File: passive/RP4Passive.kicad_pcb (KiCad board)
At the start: 2 copper layers, 30.4 x 59.4 mm, 8 parts, among them M1 Noctua

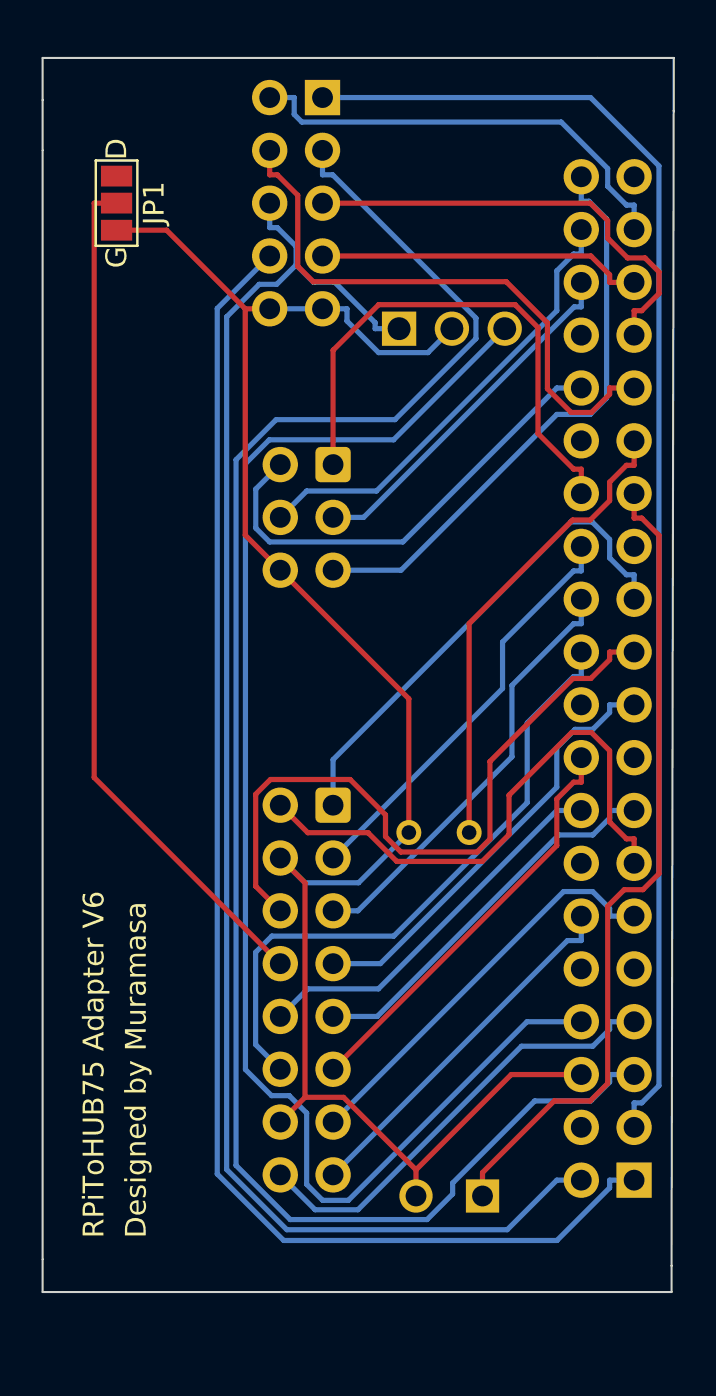
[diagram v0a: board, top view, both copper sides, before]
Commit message: version 7
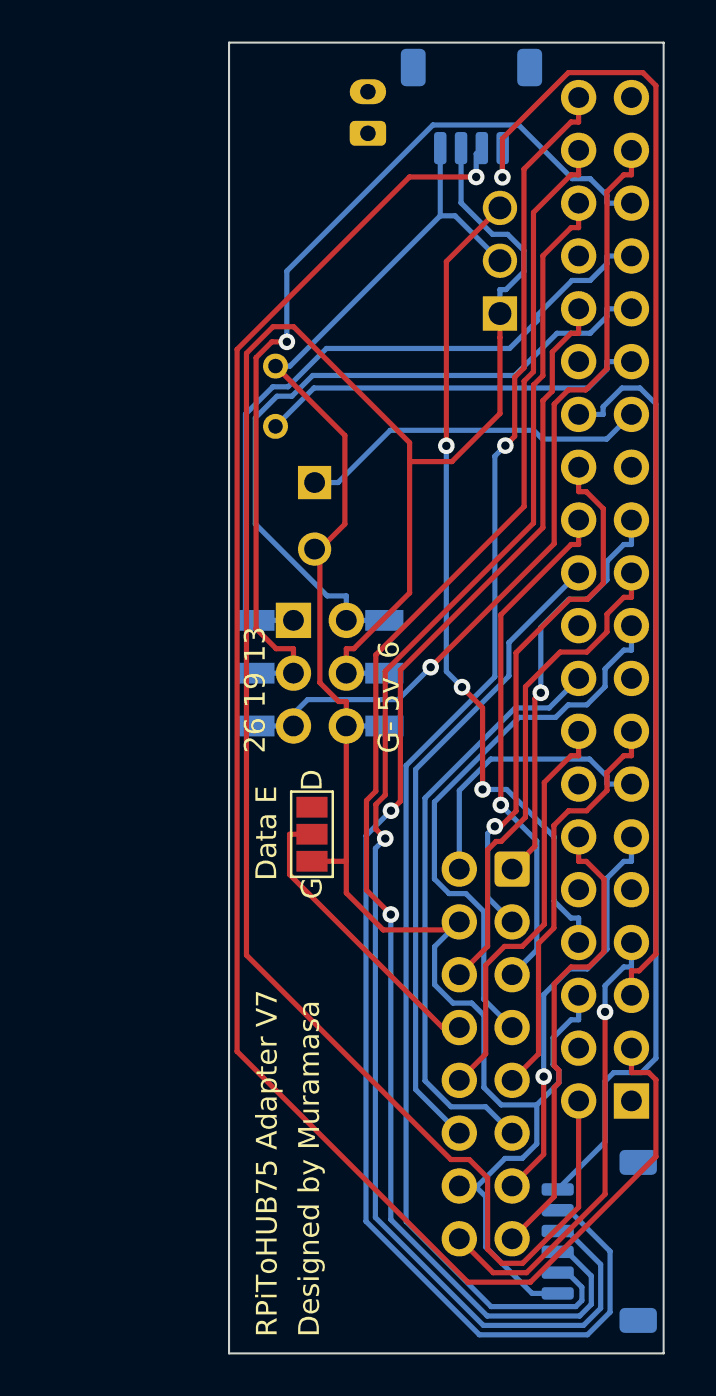
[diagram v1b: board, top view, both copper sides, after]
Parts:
- added J1: Conn_01x01, Custom:raspberrypi_2_3, B.Cu at (113.9, 81.5)
- added J2: Conn_01x02_Socket, Custom:JST_PH_S2B-PH-K_1x02_P2.00mm_Horizontal, B.Cu at (151.5, 59.1)
- added SCD30: Conn_01x04_Socket, Custom:STEMMA QT 1x04, B.Cu at (156.5, 57.8)
- GPIO1: value 02x05 -> 02x03; footprint Connector_PinHeader_2.54mm:PinHeader_2x05_P2.54mm_Horizontal -> Custom:GPIO Header
- HUB1: footprint Connector_IDC:IDC-Header_2x08_P2.54mm_Horizontal -> Custom:HUB75
- IO1: footprint Connector_IDC:IDC-Header_2x03_P2.54mm_Horizontal -> Custom:JST_SH_SM06B-SRSS-TB_1x06-1MP_P1.00mm_Horizontal
- RPiGPIO1: footprint Connector_PinSocket_2.54mm:PinSocket_2x20_P2.54mm_Vertical -> Custom:RPi GPIO
- moved IO1 39.5 mm to (162.7, 112.4), turned to -90 degrees
- moved BZ1 35.3 mm to (149.0, 75.9), turned to -90 degrees
- moved JP1 31.8 mm to (148.8, 92.8)
- moved GPIO1 27.7 mm to (149.2, 85.1)
- moved S1 21.6 mm to (147.1, 73.2), turned to 90 degrees
- moved HUB1 9.14 mm to (158.5, 94.5)
- moved M1 4.91 mm to (157.9, 67.8), turned to -90 degrees
- moved RPiGPIO1 3.81 mm to (164.2, 105.7)
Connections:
- GPIO1 pad 1: GPIO 2 -> GPIO 13
- GPIO1 pad 2: GPIO 26 -> GPIO 6
- GPIO1 pad 3: GPIO 3 -> GPIO 19
- GPIO1 pad 4: GPIO 6 -> 5v
- GPIO1 pad 5: GPIO 13 -> GPIO 26
- GPIO1 pad 6: 5v -> Net-(BZ1-+)
- RPiGPIO1 pad 1: 3.3v -> unconnected-(RPiGPIO1-Pin_1-Pad1)
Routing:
- net 3.3v: track 68.0 -> 0.00 mm
- net IO3: track 17.3 -> 71.6 mm, vias 0 -> 1
- net IO4: track 22.0 -> 71.6 mm, vias 0 -> 1
- net IO2: track 22.5 -> 69.1 mm, vias 0 -> 1
- net IO5: track 27.9 -> 70.1 mm, vias 0 -> 1
- net 5v: track 74.7 -> 105.6 mm
- net GPIO 19: track 15.7 -> 44.7 mm, vias 0 -> 1
- net FAN: track 68.6 -> 39.9 mm, vias 0 -> 3
- net GPIO 3: track 83.9 -> 56.7 mm, vias 0 -> 1
- net Net-(HUB1-Pin_8): track 41.4 -> 14.2 mm
- net BUZZ: track 39.6 -> 16.9 mm
- net IO1: track 25.8 -> 45.3 mm
- net GPIO 2: track 64.5 -> 83.6 mm, vias 0 -> 1
- net GPIO 26: track 21.8 -> 39.8 mm, vias 0 -> 1
- net G1: track 27.1 -> 13.4 mm
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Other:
- board size 30.4 x 59.4 mm -> 20.9 x 63 mm
- board text added: "26 19 13 G- 5v 6"
- board text added: "RPiToHUB75 Adapter V7"
- board text removed: "RPiToHUB75 Adapter V6"

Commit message: update image
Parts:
- J2: value Conn_01x02_Socket -> 1x02
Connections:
- J2 pad 1: unconnected-(J2-Pin_1-Pad1) -> 5v
- J2 pad 2: unconnected-(J2-Pin_2-Pad2) -> Net-(BZ1-+)
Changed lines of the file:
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@@
   (net 41 "5v")
   (net 42 "unconnected-(RPiGPIO1-Pin_1-Pad1)")
-  (net 43 "unconnected-(J2-Pin_1-Pad1)")
-  (net 44 "unconnected-(J2-Pin_2-Pad2)")
   (footprint "Jumper:SolderJumper-3_P1.3mm_Open_Pad1.0x1.5mm_NumberLabels" (layer "F.Cu")
     (at 148.844 92.837 -90)
@@
       (stroke (width 0.05) (type default)) (fill none) (layer "B.CrtYd"))
     (model "C:/Users/Admin/Downloads/RASPBERRY_PI_5.STEP/RASPBERRY_PI_5.STEP"
-      (offset (xyz 10 -24.5 12.5))
+      (opacity 0.0000)      (offset (xyz 10 -24.5 12.5))
       (scale (xyz 1 1 1))
       (rotate (xyz 90 0 0))
     )
     (model "C:/Users/Admin/Downloads/black-aluminum-heatsink-for-raspberry-pi-1.snapshot.3/Heat sink Al.step"
-      (offset (xyz 0.5 -19 7.5))
+      (opacity 0.0000)      (offset (xyz 0.5 -19 7.5))
       (scale (xyz 1 1 1))
       (rotate (xyz 90 0 0))
@@
         (effects (font (size 1 1) (thickness 0.15)) (justify mirror))
     )
-    (fp_text value "Conn_01x02_Socket" (at 1 -7.45 90) (layer "B.Fab") hide
+    (fp_text value "1x02" (at 1 -7.45 90) (layer "B.Fab") hide
         (effects (font (size 1 1) (thickness 0.15)) (justify mirror))
     )
@@
       (stroke (width 0.1) (type solid)) (layer "B.Fab"))
     (pad "1" thru_hole roundrect (at 0 0 90) (size 1.2 1.75) (drill 0.75) (layers "*.Cu" "*.Mask") (roundrect_rratio 0.208333)
-      (net 43 "unconnected-(J2-Pin_1-Pad1)") (pinfunction "Pin_1") (pintype "passive+no_connect"))
+      (net 41 "5v") (pinfunction "Pin_1") (pintype "passive"))
     (pad "2" thru_hole oval (at 2 0 90) (size 1.2 1.75) (drill 0.75) (layers "*.Cu" "*.Mask")
-      (net 44 "unconnected-(J2-Pin_2-Pad2)") (pinfunction "Pin_2") (pintype "passive+no_connect"))
+      (net 2 "Net-(BZ1-+)") (pinfunction "Pin_2") (pintype "passive"))
     (model "${KICAD6_3DMODEL_DIR}/Connector_JST.3dshapes/JST_PH_S2B-PH-K_1x02_P2.00mm_Horizontal.wrl"
       (offset (xyz 0 0 0))
